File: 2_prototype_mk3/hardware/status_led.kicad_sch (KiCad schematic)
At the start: 2 parts

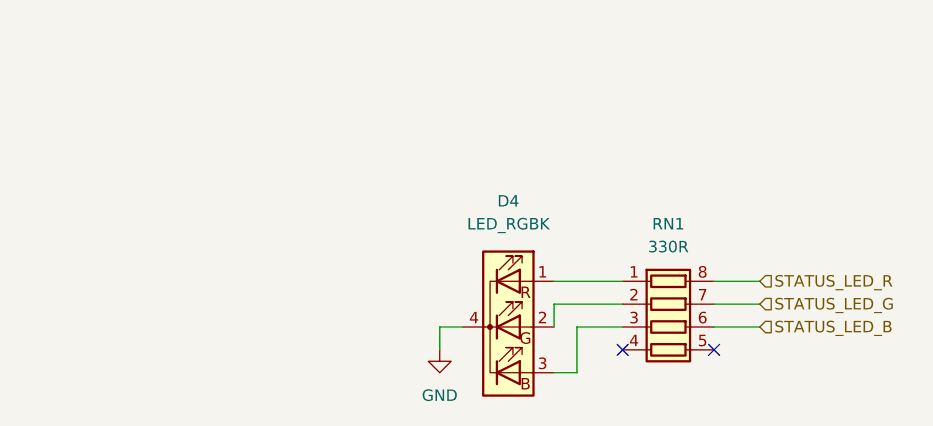
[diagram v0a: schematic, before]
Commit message: MKIII design refinements
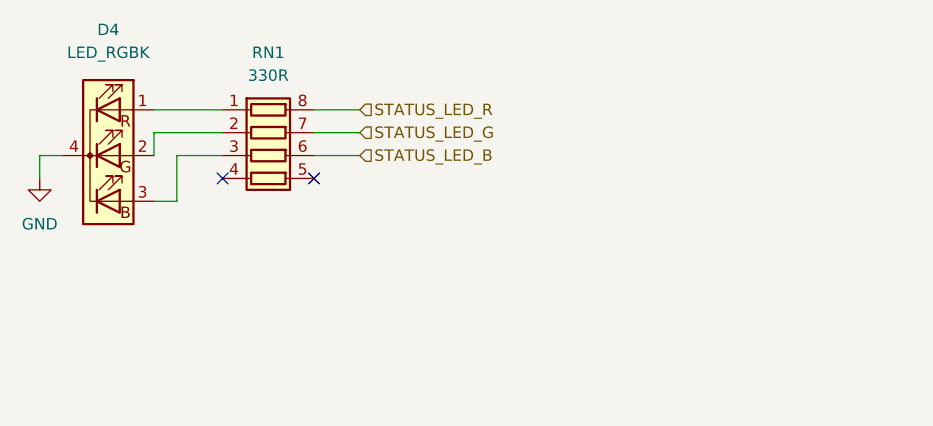
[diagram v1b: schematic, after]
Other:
- title: (none) -> Status LED
- moved on the sheet: D4, RN1
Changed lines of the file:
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@@
 	(generator "eeschema")
 	(generator_version "9.0")
-	(paper "A4")
+	(paper "A5")
+	(title_block
+		(title "Status LED")
+	)
 	(no_connect
-		(at 144.78 92.71)
+		(at 100.33 73.66)
 	)
 	(no_connect
-		(at 154.94 92.71)
-	)
-	(wire
-		(pts
-			(xy 154.94 87.63) (xy 160.02 87.63)
-		)
-		(stroke
-			(width 0)
-			(type default)
-		)
-	)
-	(wire
-		(pts
-			(xy 139.7 95.25) (xy 137.16 95.25)
-		)
-		(stroke
-			(width 0)
-			(type default)
-		)
-	)
-	(wire
-		(pts
-			(xy 144.78 90.17) (xy 139.7 90.17)
-		)
-		(stroke
-			(width 0)
-			(type default)
-		)
-	)
-	(wire
-		(pts
-			(xy 154.94 85.09) (xy 160.02 85.09)
-		)
-		(stroke
-			(width 0)
-			(type default)
-		)
-	)
-	(wire
-		(pts
-			(xy 139.7 90.17) (xy 139.7 95.25)
-		)
-		(stroke
-			(width 0)
-			(type default)
-		)
-	)
-	(wire
-		(pts
-			(xy 137.16 87.63) (xy 144.78 87.63)
-		)
-		(stroke
-			(width 0)
-			(type default)
-		)
-	)
-	(wire
-		(pts
-			(xy 124.46 90.17) (xy 124.46 92.71)
-		)
-		(stroke
-			(width 0)
-			(type default)
-		)
-	)
-	(wire
-		(pts
-			(xy 137.16 90.17) (xy 137.16 87.63)
-		)
-		(stroke
-			(width 0)
-			(type default)
-		)
-	)
-	(wire
-		(pts
-			(xy 154.94 90.17) (xy 160.02 90.17)
-		)
-		(stroke
-			(width 0)
-			(type default)
-		)
-	)
-	(wire
-		(pts
-			(xy 127 90.17) (xy 124.46 90.17)
-		)
-		(stroke
-			(width 0)
-			(type default)
-		)
-	)
-	(wire
-		(pts
-			(xy 137.16 85.09) (xy 144.78 85.09)
+		(at 110.49 73.66)
+	)
+	(wire
+		(pts
+			(xy 110.49 68.58) (xy 115.57 68.58)
+		)
+		(stroke
+			(width 0)
+			(type default)
+		)
+	)
+	(wire
+		(pts
+			(xy 95.25 76.2) (xy 92.71 76.2)
+		)
+		(stroke
+			(width 0)
+			(type default)
+		)
+	)
+	(wire
+		(pts
+			(xy 100.33 71.12) (xy 95.25 71.12)
+		)
+		(stroke
+			(width 0)
+			(type default)
+		)
+	)
+	(wire
+		(pts
+			(xy 110.49 66.04) (xy 115.57 66.04)
+		)
+		(stroke
+			(width 0)
+			(type default)
+		)
+	)
+	(wire
+		(pts
+			(xy 95.25 71.12) (xy 95.25 76.2)
+		)
+		(stroke
+			(width 0)
+			(type default)
+		)
+	)
+	(wire
+		(pts
+			(xy 92.71 68.58) (xy 100.33 68.58)
+		)
+		(stroke
+			(width 0)
+			(type default)
+		)
+	)
+	(wire
+		(pts
+			(xy 80.01 71.12) (xy 80.01 73.66)
+		)
+		(stroke
+			(width 0)
+			(type default)
+		)
+	)
+	(wire
+		(pts
+			(xy 92.71 71.12) (xy 92.71 68.58)
+		)
+		(stroke
+			(width 0)
+			(type default)
+		)
+	)
+	(wire
+		(pts
+			(xy 110.49 71.12) (xy 115.57 71.12)
+		)
+		(stroke
+			(width 0)
+			(type default)
+		)
+	)
+	(wire
+		(pts
+			(xy 82.55 71.12) (xy 80.01 71.12)
+		)
+		(stroke
+			(width 0)
+			(type default)
+		)
+	)
+	(wire
+		(pts
+			(xy 92.71 66.04) (xy 100.33 66.04)
 		)
 		(stroke
@@
 	(hierarchical_label "STATUS_LED_G"
 		(shape input)
-		(at 160.02 87.63 0)
+		(at 115.57 68.58 0)
 		(effects
 			(font
@@
 	(hierarchical_label "STATUS_LED_R"
 		(shape input)
-		(at 160.02 85.09 0)
+		(at 115.57 66.04 0)
 		(effects
 			(font
@@
 	(hierarchical_label "STATUS_LED_B"
 		(shape input)
-		(at 160.02 90.17 0)
+		(at 115.57 71.12 0)
 		(effects
 			(font
@@
 	(symbol
 		(lib_id "Device:LED_RGBK")
-		(at 132.08 90.17 0)
+		(at 87.63 71.12 0)
 		(unit 1)
 		(exclude_from_sim no)
@@
 		(fields_autoplaced yes)
 		(property "Reference" "D4"
-			(at 132.08 76.2 0)
+			(at 87.63 57.15 0)
 			(effects
 				(font
@@
 		)
 		(property "Value" "LED_RGBK"
-			(at 132.08 78.74 0)
+			(at 87.63 59.69 0)
 			(effects
 				(font
@@
 		)
 		(property "Footprint" "LED_THT:LED_D5.0mm-4_RGB"
-			(at 132.08 91.44 0)
+			(at 87.63 72.39 0)
 			(effects
 				(font
@@
 		)
 		(property "Datasheet" "~"
-			(at 132.08 91.44 0)
+			(at 87.63 72.39 0)
 			(effects
 				(font
@@
 		)
 		(property "Description" "RGB LED, red/green/blue/cathode"
-			(at 132.08 90.17 0)
+			(at 87.63 71.12 0)
 			(effects
 				(font
@@
 	(symbol
 		(lib_id "power:GND")
-		(at 124.46 92.71 0)
+		(at 80.01 73.66 0)
 		(unit 1)
 		(exclude_from_sim no)
@@
 		(fields_autoplaced yes)
 		(property "Reference" "#PWR06"
-			(at 124.46 99.06 0)
+			(at 80.01 80.01 0)
 			(effects
 				(font
@@
 		)
 		(property "Value" "GND"
-			(at 124.46 97.79 0)
+			(at 80.01 78.74 0)
 			(effects
 				(font
@@
 		)
 		(property "Footprint" ""
-			(at 124.46 92.71 0)
+			(at 80.01 73.66 0)
 			(effects
 				(font
@@
 		)
 		(property "Datasheet" ""
-			(at 124.46 92.71 0)
+			(at 80.01 73.66 0)
 			(effects
 				(font
@@
 		)
 		(property "Description" "Power symbol creates a global label with name \"GND\" , ground"
-			(at 124.46 92.71 0)
+			(at 80.01 73.66 0)
 			(effects
 				(font
@@
 	(symbol
 		(lib_id "Device:R_Pack04")
-		(at 149.86 90.17 270)
+		(at 105.41 71.12 270)
 		(unit 1)
 		(exclude_from_sim no)
@@
 		(fields_autoplaced yes)
 		(property "Reference" "RN1"
-			(at 149.86 78.74 90)
+			(at 105.41 59.69 90)
 			(effects
 				(font
@@
 		)
 		(property "Value" "330R"
-			(at 149.86 81.28 90)
+			(at 105.41 62.23 90)
 			(effects
 				(font
@@
 		)
 		(property "Footprint" "Resistor_SMD:R_Array_Convex_4x0603"
-			(at 149.86 97.155 90)
+			(at 105.41 78.105 90)
 			(effects
 				(font
@@
 		)
 		(property "Datasheet" "~"
-			(at 149.86 90.17 0)
+			(at 105.41 71.12 0)
 			(effects
 				(font
@@
 		)
 		(property "Description" "4 resistor network, parallel topology"
-			(at 149.86 90.17 0)
-			(effects
-				(font
+			(at 105.41 71.12 0)
+			(effects
+				(font
